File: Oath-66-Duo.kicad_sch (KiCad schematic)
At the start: 67 parts, among them U1 Arduino_Pro_Micro

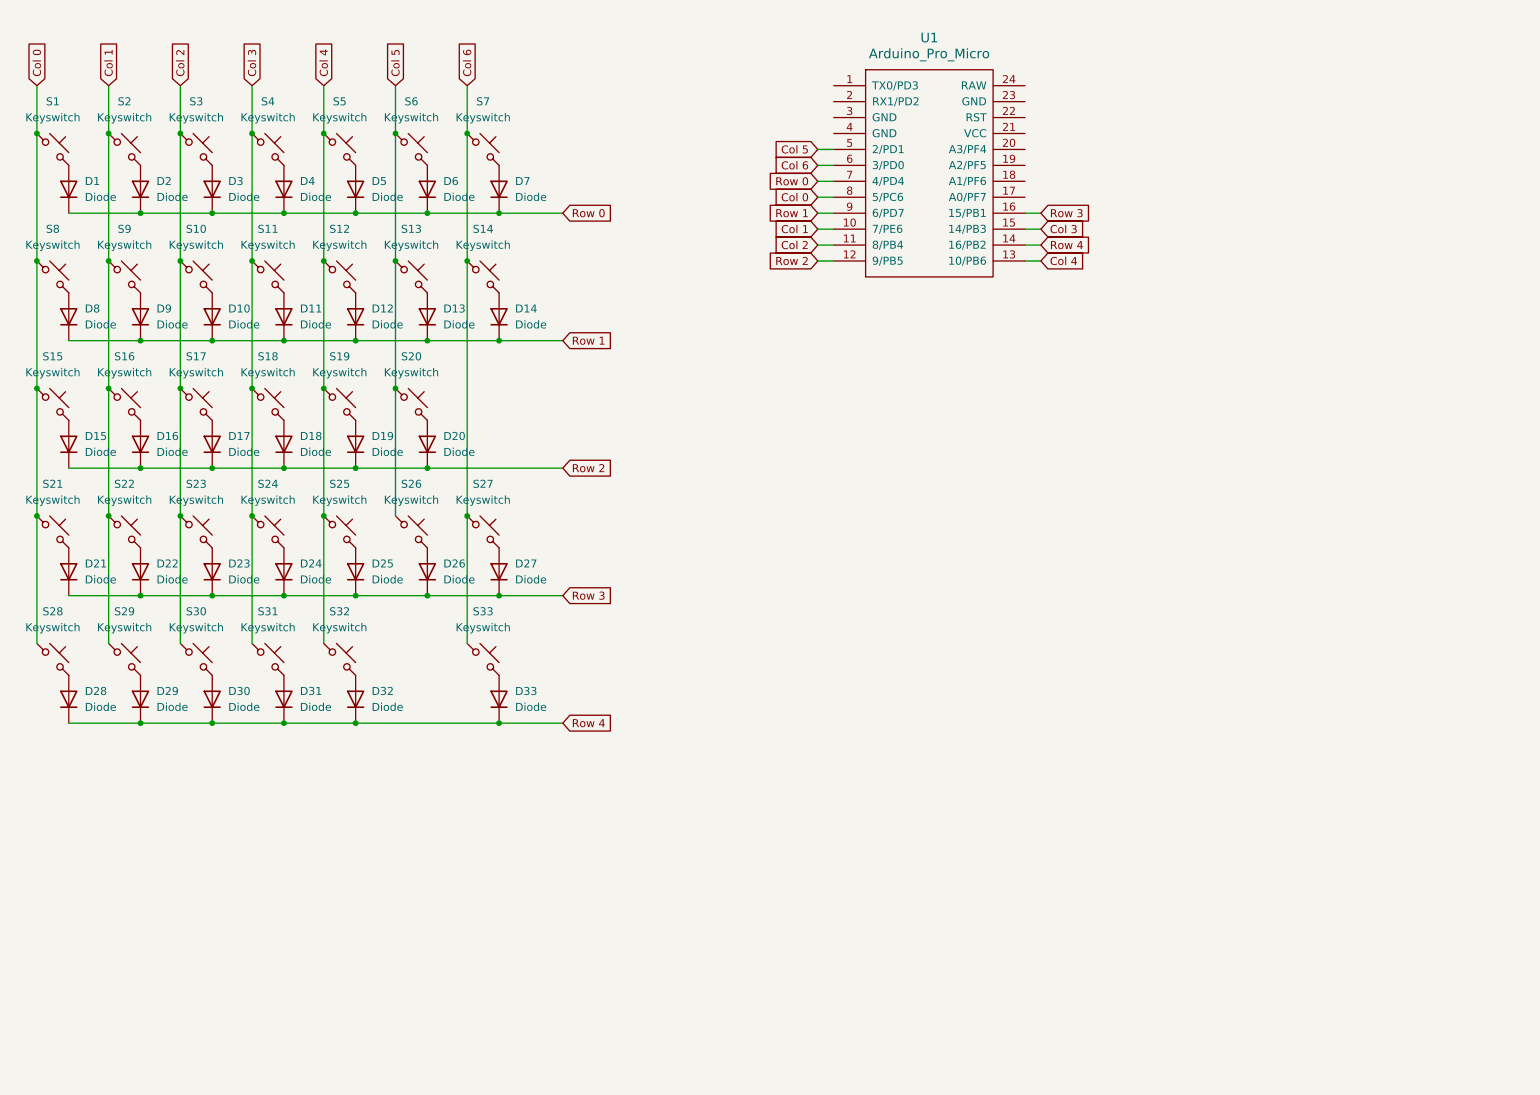
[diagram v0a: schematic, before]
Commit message: Sub-Schematic Updated
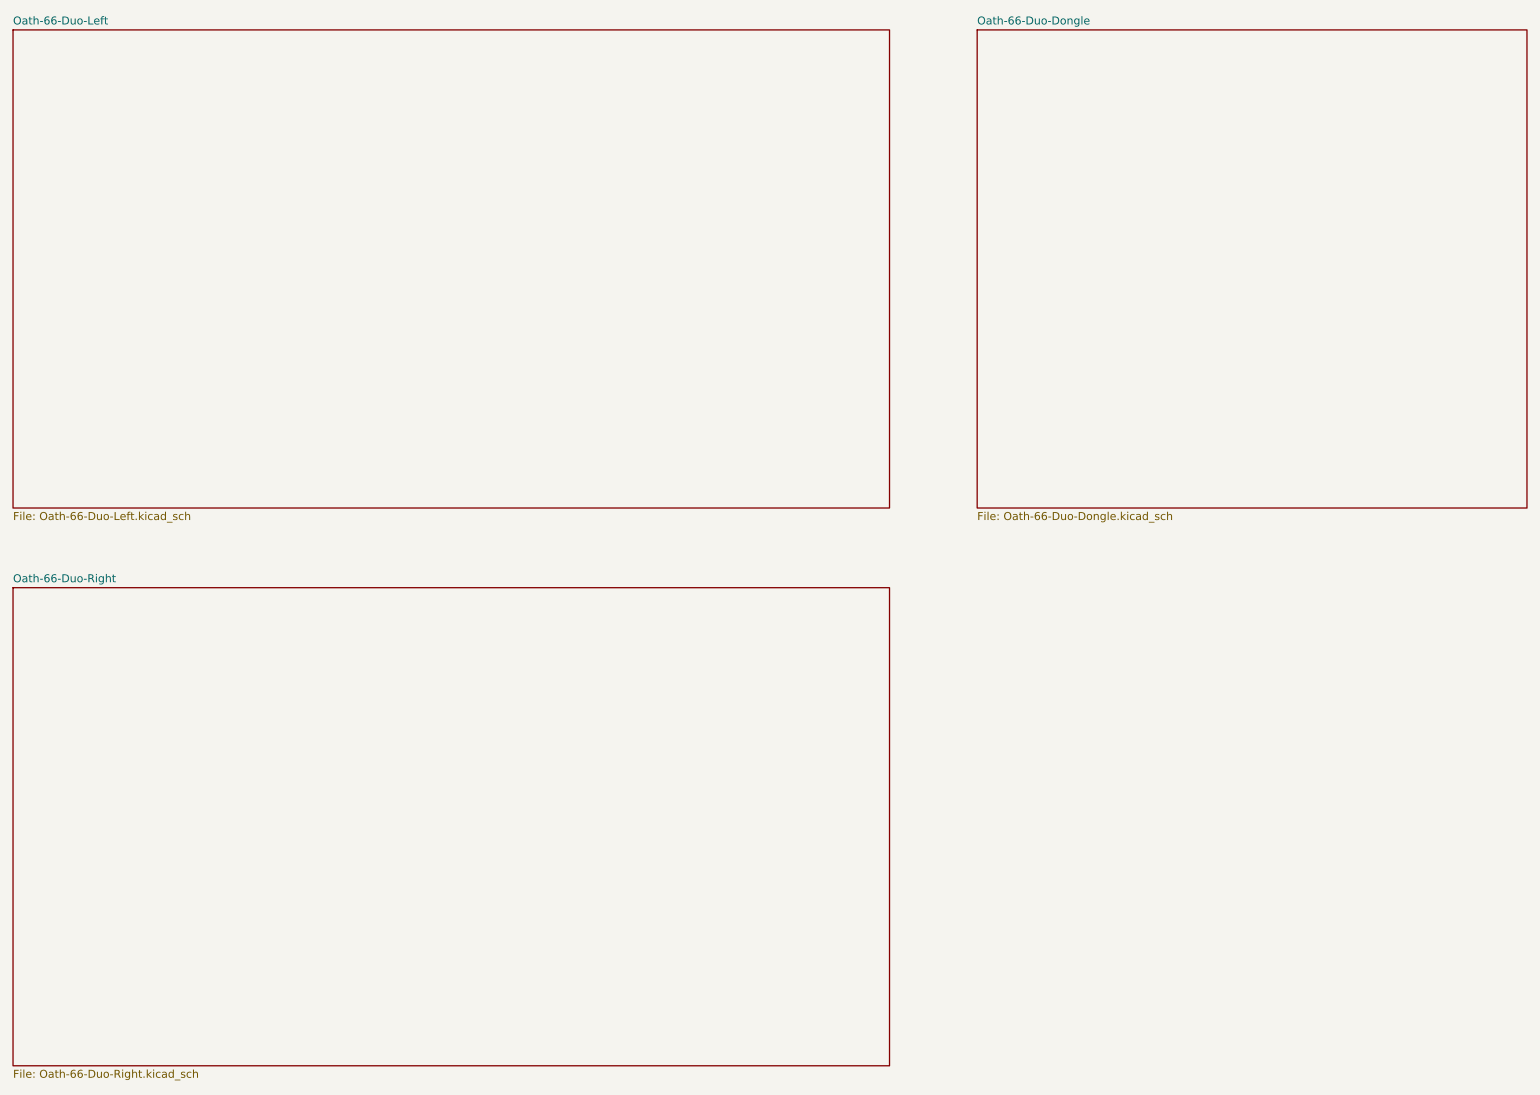
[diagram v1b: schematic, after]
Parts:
- removed D1, D10, D11, D12, D13, D14, D15, D16, D17, D18, D19, D2, D20, D21, D22, D23, D24, D25, D26, D27, D28, D29, D3, D30, D31, D32, D33, D4, D5, D6, D7, D8, D9: Diode, ScottoKeebs_Components:Diode_SOD-123, symbol ScottoKeebs:Placeholder_Diode
- removed S1, S10, S11, S12, S13, S14, S15, S16, S17, S18, S19, S2, S20, S21, S22, S23, S24, S25, S26, S28, S29, S3, S30, S31, S33, S4, S5, S6, S7, S8, S9: Keyswitch, ScottoKeebs_Hotswap:Hotswap_MX_1.00u, symbol ScottoKeebs:Placeholder_Keyswitch
- removed S27: Keyswitch, ScottoKeebs_Hotswap:Hotswap_MX_2.00u_90deg, symbol ScottoKeebs:Placeholder_Keyswitch
- removed S32: Keyswitch, ScottoKeebs_Hotswap:Hotswap_MX_2.00u, symbol ScottoKeebs:Placeholder_Keyswitch
- removed U1: Arduino_Pro_Micro, ScottoKeebs_MCU:Arduino_Pro_Micro, symbol ScottoKeebs:MCU_Arduino_Pro_Micro
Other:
- added sheet Oath-66-Duo-Dongle (Oath-66-Duo-Dongle.kicad_sch)
- added sheet Oath-66-Duo-Left (Oath-66-Duo-Left.kicad_sch)
- added sheet Oath-66-Duo-Right (Oath-66-Duo-Right.kicad_sch)
